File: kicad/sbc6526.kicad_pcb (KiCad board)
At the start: 4 copper layers, 100 x 100 mm, 59 parts, among them P1 2k, P2 5k, SW1 UP, SW2 DOWN, SW3 OK, SW4 CANCEL, SW5 RESET, U1 6526, U10 74AC138, U11 74ACT245, U2 W65C22SxP, U3 W65C02SxP, U4 IS61C1024AL-12KLI, U5 74HC595, U6 74HC595, U7 74AC74, U8 74AC14, U9 74AC139, Y1 20M

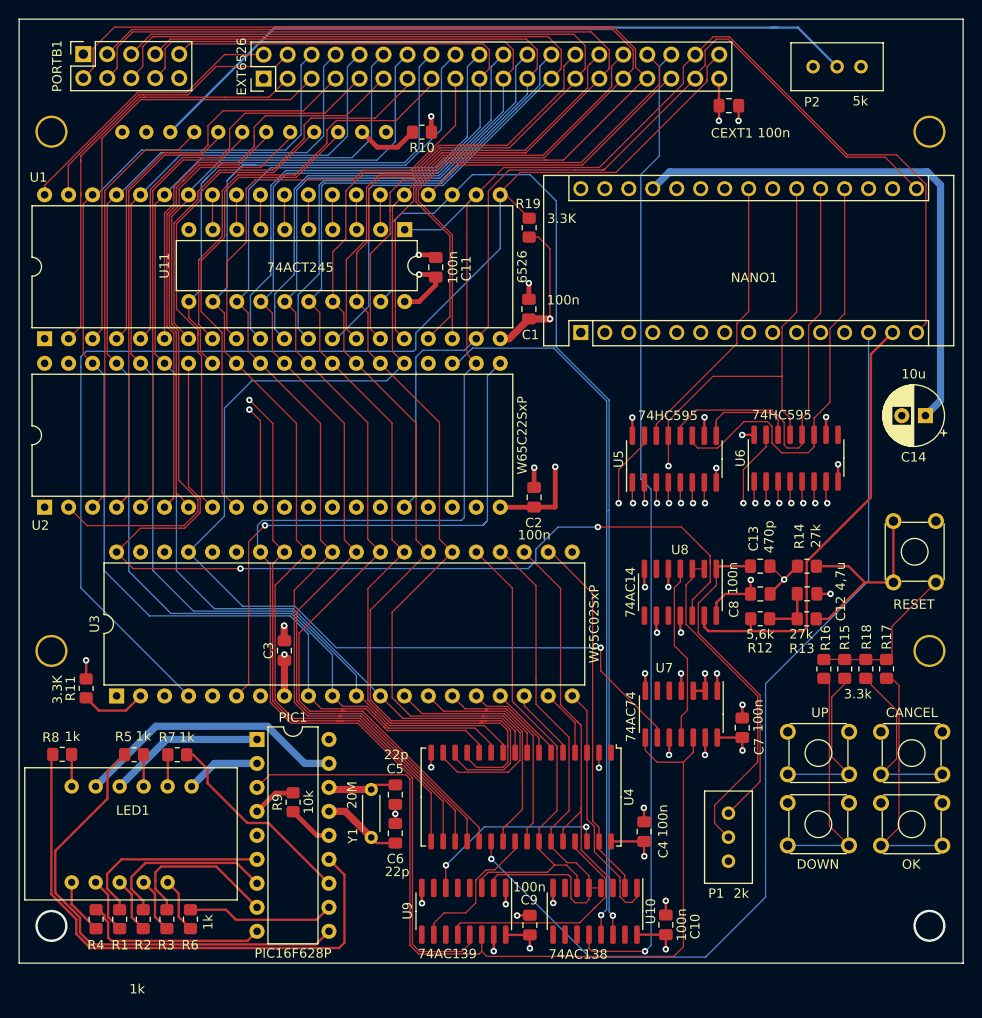
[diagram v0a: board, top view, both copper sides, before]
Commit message: v2.0
Production ready
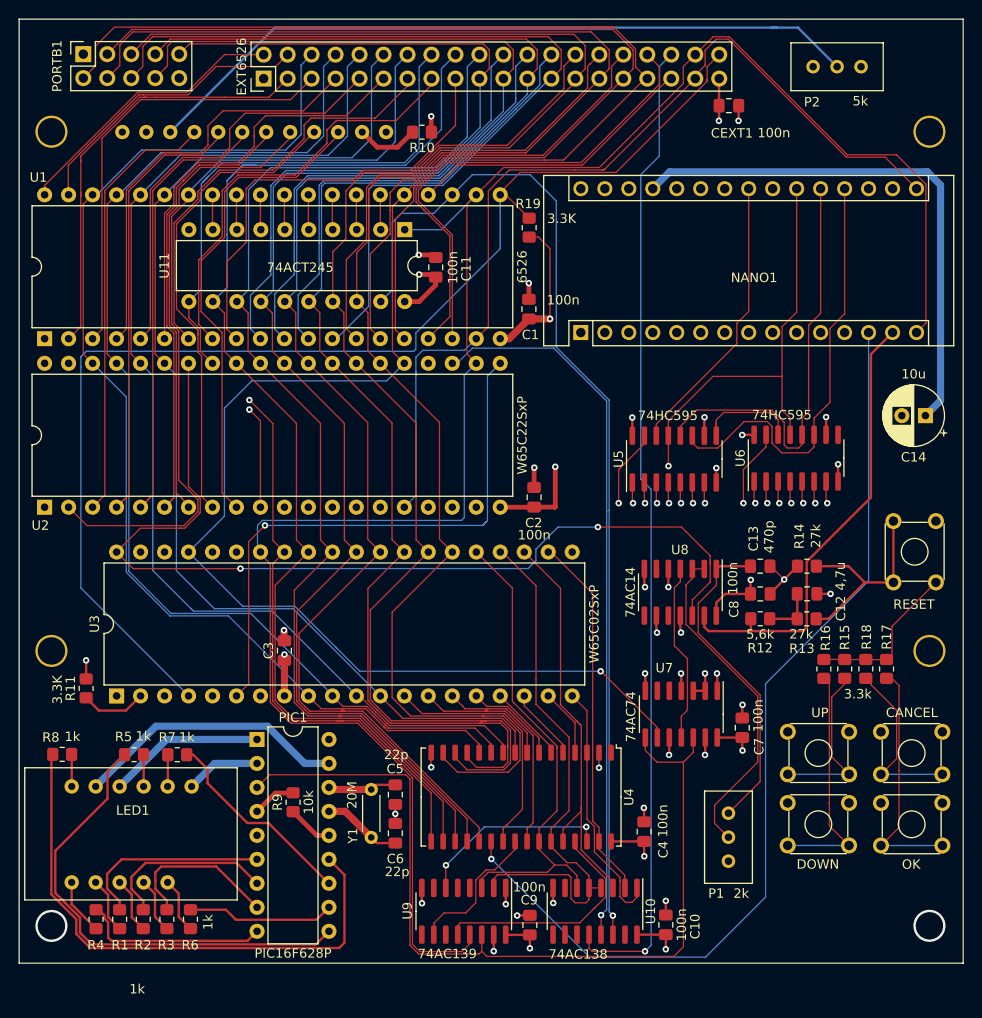
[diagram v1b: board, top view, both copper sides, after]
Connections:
- net D0 renamed /D0
- net D1 renamed /D1
- net D2 renamed /D2
- net D3 renamed /D3
- net D4 renamed /D4
- net D5 renamed /D5
- net D6 renamed /D6
- net D7 renamed /D7
- LCD1 pad : GND -> (no net)
- U4 pad 1: (no net) -> no_connect_146
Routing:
- net /A0: track 177.9 -> 172.8 mm
- net /A1: track 167.4 -> 165.2 mm
- net /PHI2: track 148.8 -> 147.5 mm
- net /A2: track 163.5 -> 162.6 mm
